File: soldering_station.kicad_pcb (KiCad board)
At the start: 2 copper layers, 42.4 x 23 mm, 71 parts, among them IC1 ATMEGA8A-P, K1 dec in, K2 dec out, P1 17v, P10 disp in, P2 220v, P3 24v|220v, P4 solder, P5 thermocouple, P6 Fan, P7 thermocouple, P8 Heater, P9 disp out, Q1 КТ313Б, Q2 КТ313Б, Q3 КТ313Б, Q4 КТ815А, SW2 Enc, U1 TL072, U2 MOC3023M, U3 MOC3023M, U4 LM7805CT

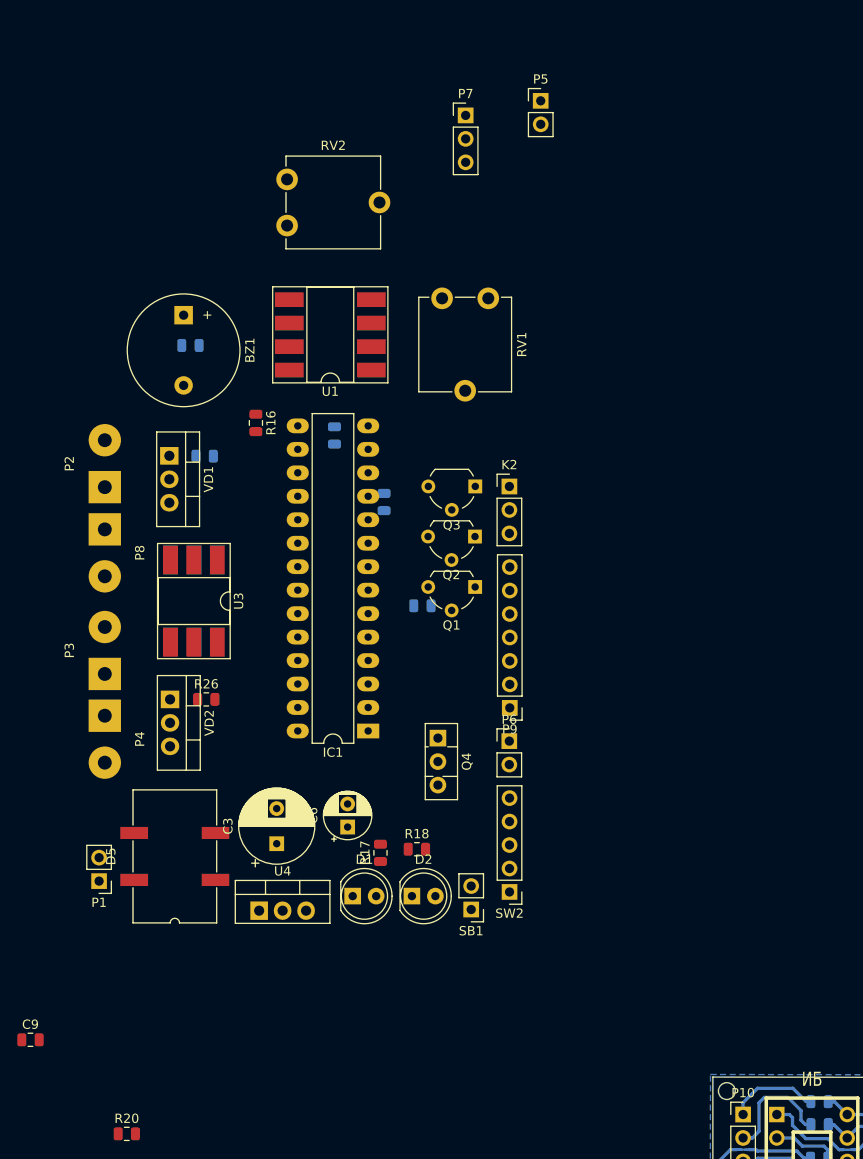
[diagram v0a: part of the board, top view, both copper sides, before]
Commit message: Display PCB
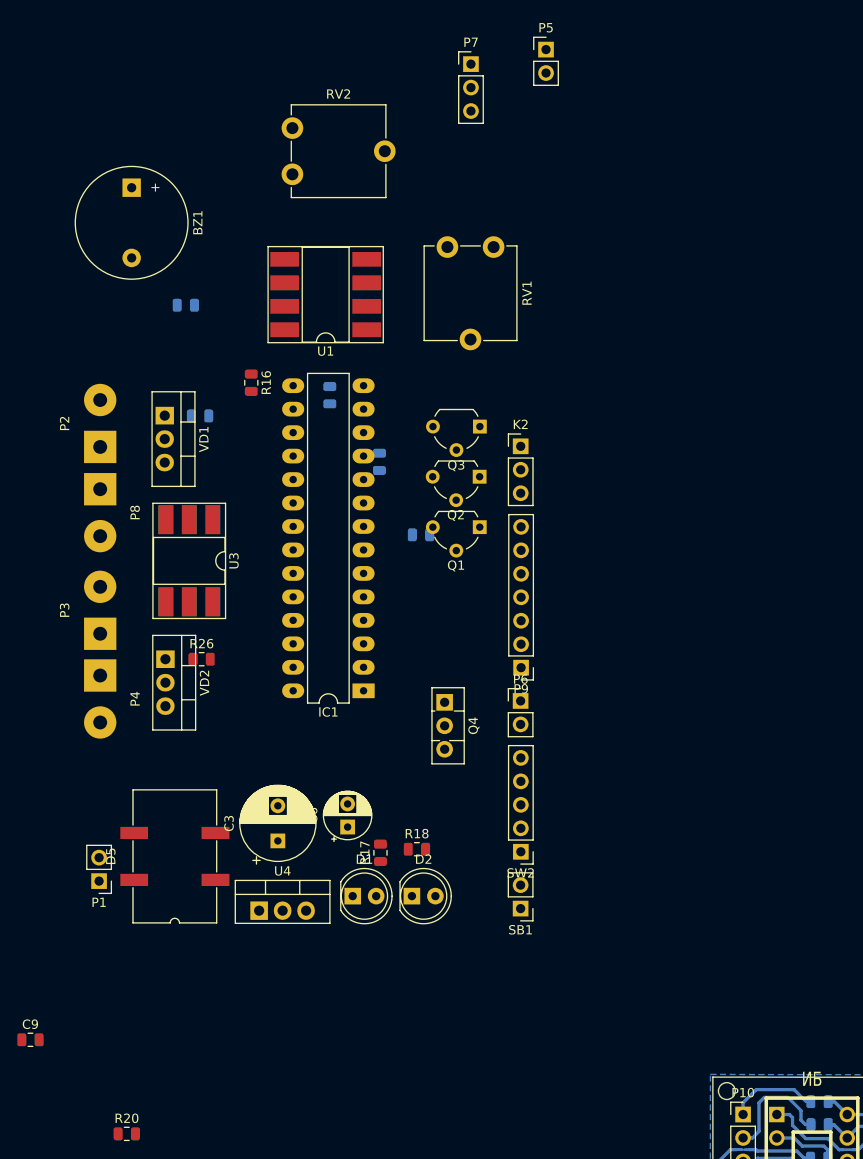
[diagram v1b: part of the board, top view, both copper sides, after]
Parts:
- moved BZ1 14.9 mm to (165.3, 27.6)
- moved R10 7.68 mm to (196.7, 65.1)
- moved Q1 6.49 mm to (203.0, 64.3)
- moved Q2 6.49 mm to (203.0, 58.9)
- moved Q3 6.49 mm to (203.0, 53.4)
- moved P5 5.58 mm to (210.2, 12.6)
- moved P7 5.58 mm to (202.1, 14.2)
- moved RV2 5.58 mm to (182.8, 26.1)
- moved RV1 5.58 mm to (199.5, 34.0)
- moved SB1 5.35 mm to (207.4, 105.6)
- moved K2 4.52 mm to (207.5, 55.6)
- moved P6 4.52 mm to (207.4, 83.1)
- moved P9 4.52 mm to (207.5, 79.5)
- moved SW2 4.52 mm to (207.5, 99.5)
- moved P4 4.38 mm to (161.9, 80.4)
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
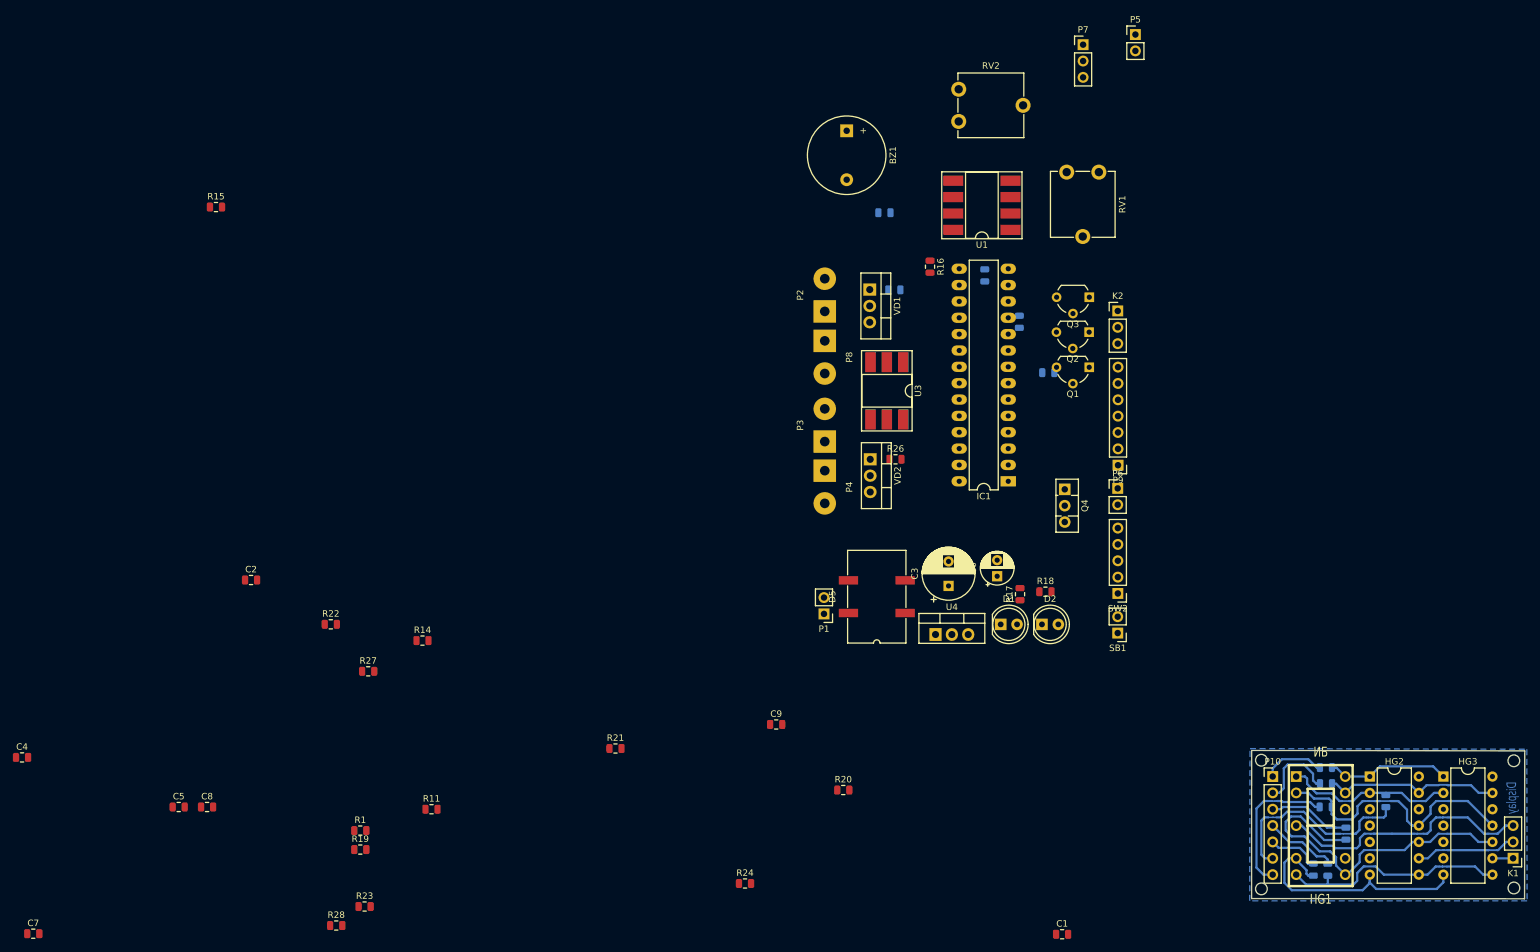
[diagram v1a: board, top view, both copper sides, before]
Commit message: Update PCB
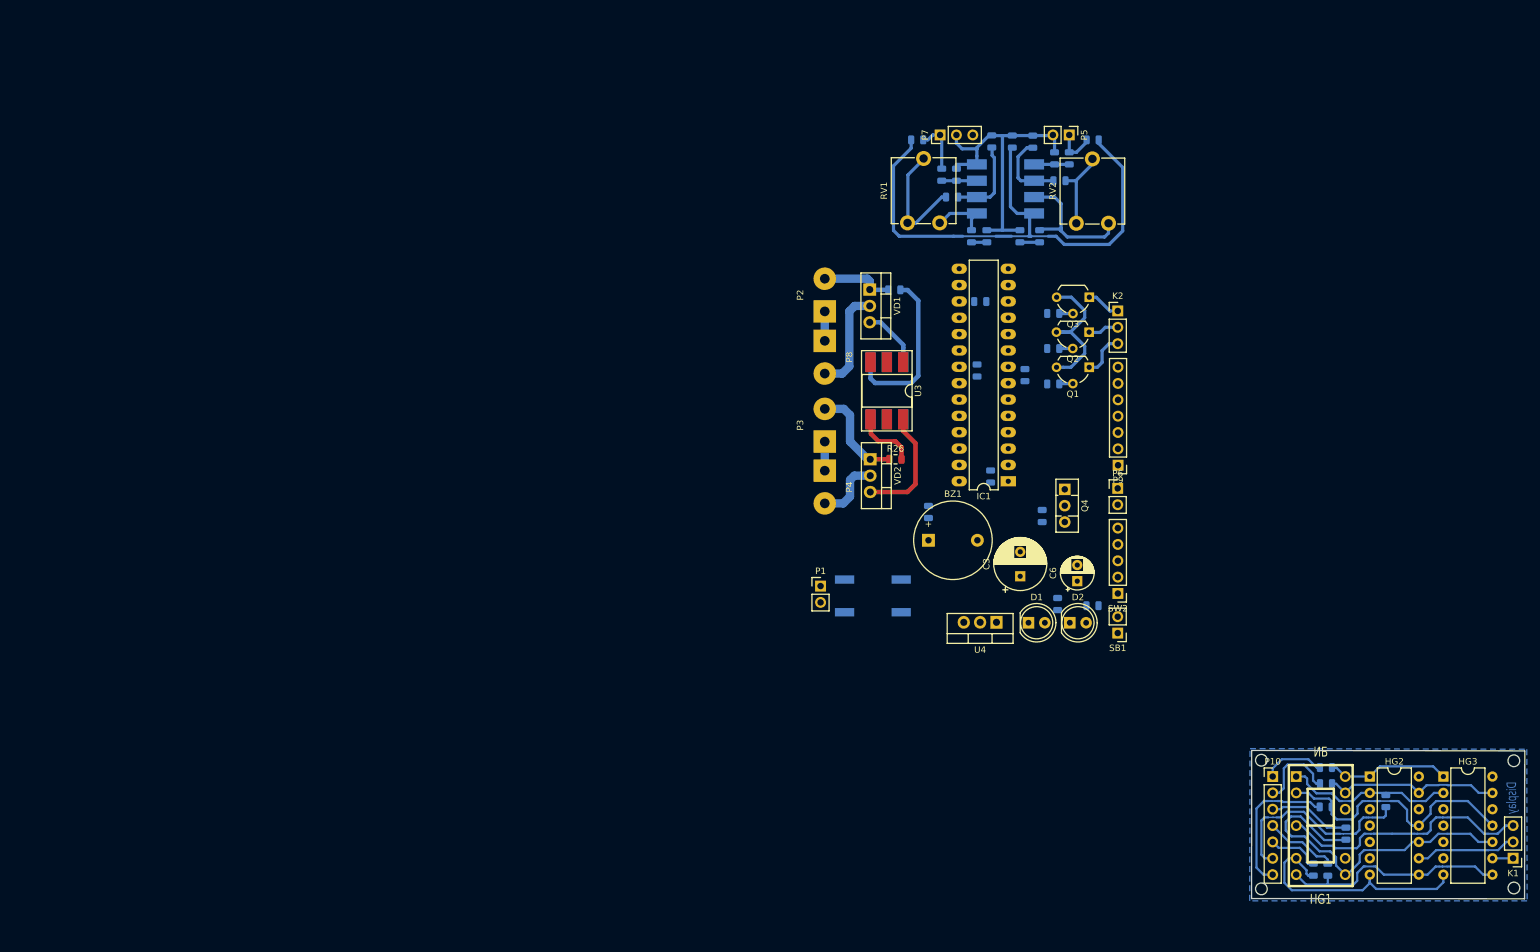
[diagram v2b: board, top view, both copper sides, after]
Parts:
- C1, C2, C4, C5, C7, C8, C9, D5, R1, R11, R14, R15, R16, R17, R18, R19, R20, R21, R22, R23, R24, R27, R28, U1: moved to B.Cu
- moved C7 176.8 mm to (193.0, 65.5), turned to 90 degrees
- moved C4 171.1 mm to (182.4, 34.4), turned to 90 degrees
- moved R28 169.4 mm to (203.6, 29.0), turned to 180 degrees
- moved C5 169.3 mm to (197.6, 31.9), turned to 90 degrees
- moved C8 162.3 mm to (191.1, 29.3), turned to 90 degrees
- moved R23 144.8 mm to (180.1, 34.4), turned to 270 degrees
- moved R19 136.8 mm to (181.7, 37.9)
- moved R22 132.3 mm to (194.3, 29.3), turned to 90 degrees
- moved C2 130.8 mm to (192.3, 44.0), turned to 90 degrees
- moved R24 123.4 mm to (199.9, 31.9), turned to 270 degrees
- moved R27 118.7 mm to (176.3, 29.0)
- moved R15 117.5 mm to (184.7, 44.0), turned to 270 degrees
- moved R11 116.1 mm to (186.1, 54.1), turned to 180 degrees
- moved R1 112.3 mm to (187.7, 81.3), turned to 90 degrees
- moved R21 112.0 mm to (198.4, 35.3), turned to 180 degrees
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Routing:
- net +5V: track 0.00 -> 108.8 mm
- net GND: track 0.00 -> 46.5 mm
- net Net-(R25-Pad2): track 0.00 -> 25.9 mm
- net Net-(R16-Pad1): track 0.00 -> 22.2 mm
- net Net-(R19-Pad1): track 0.00 -> 18.6 mm
- net Net-(U3-Pad6): track 0.00 -> 18.4 mm
- net Net-(P8-Pad2): track 0.00 -> 16.3 mm
- net Net-(P3-Pad2): track 0.00 -> 15.7 mm
- net Net-(R19-Pad2): track 0.00 -> 13.1 mm
- net Net-(R21-Pad1): track 0.00 -> 12.7 mm
- net Net-(R21-Pad2): track 0.00 -> 11.8 mm
- net Net-(P2-Pad2): track 0.00 -> 11.3 mm
- net Net-(P4-Pad2): track 0.00 -> 10.4 mm
- net Net-(R26-Pad2): track 0.00 -> 9.94 mm
- net Net-(U2-Pad6): track 0.00 -> 9.34 mm
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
